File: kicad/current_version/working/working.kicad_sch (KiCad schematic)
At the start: 4 parts, among them IC1 imsp10mpump21rs2227

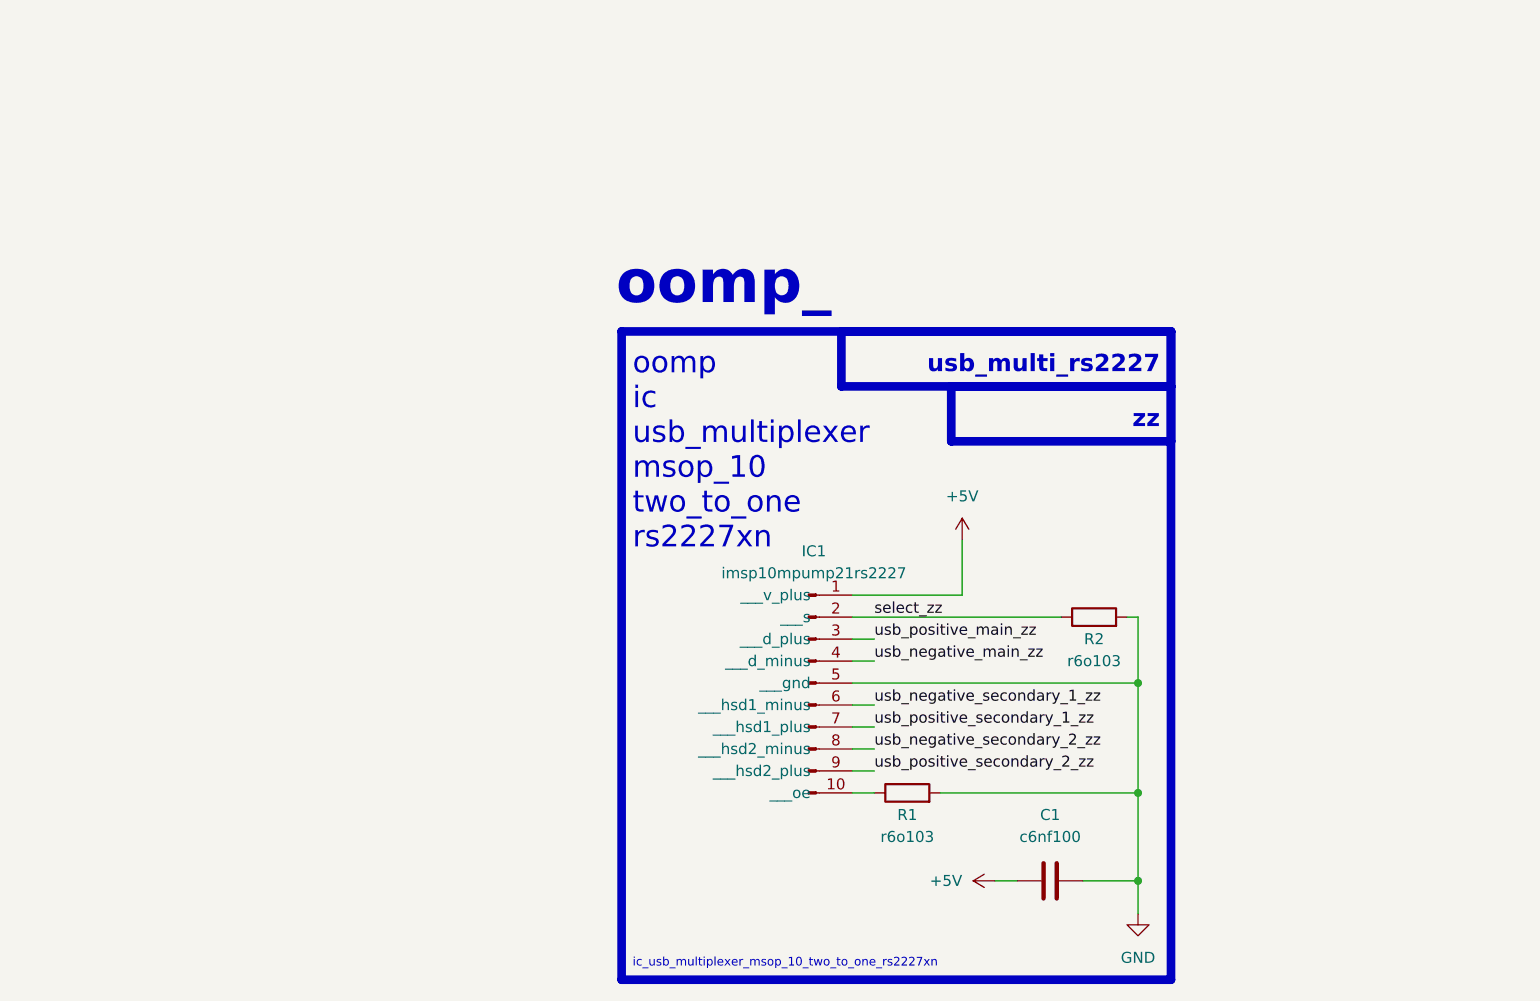
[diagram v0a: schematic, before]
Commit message: initial
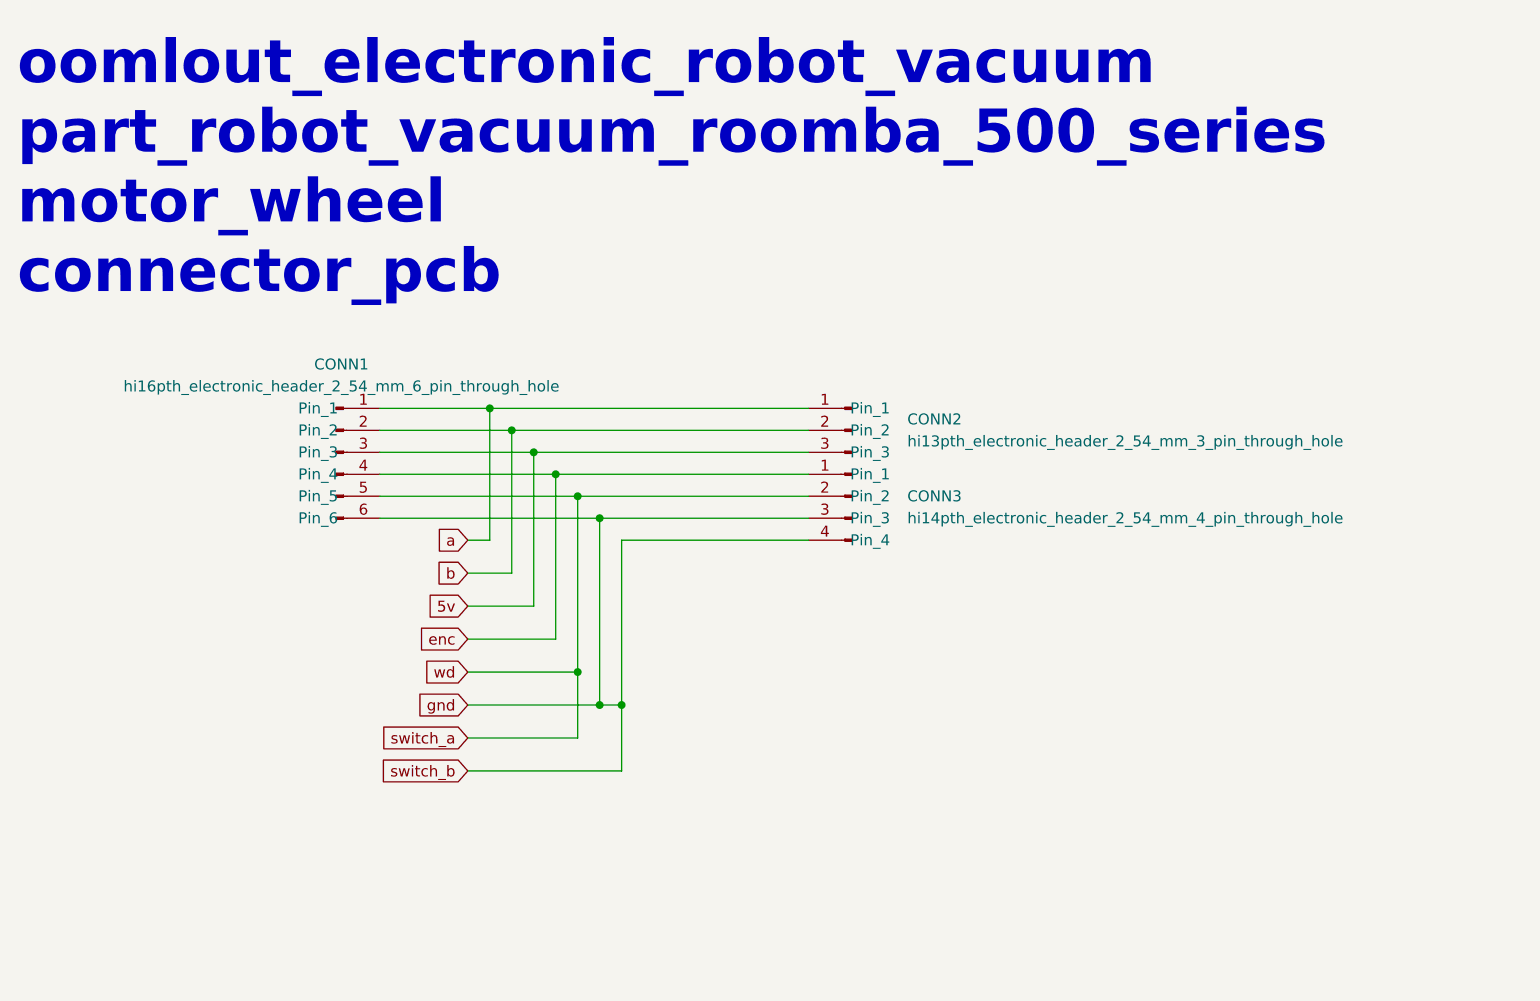
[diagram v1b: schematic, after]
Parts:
- removed C1: c6nf100, oomlout_oomp_part_footprints:c6nf100_electronic_capacitor_0603_100_nano_farad, symbol oomlout_oomp_part_symbols:c6nf100_electronic_capacitor_0603_100_nano_farad
- removed IC1: imsp10mpump21rs2227, oomlout_oomp_part_footprints:imsp10mpump21rs2227_electronic_ic_msop_10_multiplexer_usb_multiplexer_two_to_one_jiangsu_r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, symbol oomlout_oomp_part_symbols:imsp10mpump21rs2227_electronic_ic_msop_10_multiplexer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
- removed R1, R2: r6o103, oomlout_oomp_part_footprints:r6o103_electronic_resistor_0603_10000_ohm, symbol oomlout_oomp_part_symbols:r6o103_electronic_resistor_0603_10000_ohm
- added CONN1: hi16pth_electronic_header_2_54_mm_6_pin_through_h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, oomlout_oomp_part_footprints:hi16pth_electronic_header_2_54_mm_6_pin_through_hole, symbol oomp:hi16pth_electronic_header_2_54_mm_6_pin_through_hole
- added CONN2: hi13pth_electronic_header_2_54_mm_3_pin_through_h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, oomlout_oomp_part_footprints:hi13pth_electronic_header_2_54_mm_3_pin_through_hole, symbol oomp:hi13pth_electronic_header_2_54_mm_3_pin_through_hole
- added CONN3: hi14pth_electronic_header_2_54_mm_4_pin_through_h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, oomlout_oomp_part_footprints:hi14pth_electronic_header_2_54_mm_4_pin_through_hole, symbol oomp:hi14pth_electronic_header_2_54_mm_4_pin_through_hole
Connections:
- new net 5v: CONN1.3 (Pin_3), CONN2.3 (Pin_3)
- new net a: CONN1.1 (Pin_1), CONN2.1 (Pin_1)
- new net b: CONN1.2 (Pin_2), CONN2.2 (Pin_2)
- new net enc: CONN1.4 (Pin_4), CONN3.1 (Pin_1)
- new net gnd: CONN1.6 (Pin_6), CONN3.3 (Pin_3), CONN3.4 (Pin_4)
- new net switch_a: CONN1.5 (Pin_5), CONN3.2 (Pin_2)
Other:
- note added: "oomlout_electronic_robot_vacuum part_robot_vacuum_roomba_500_series motor_wheel connector_pcb"
- note removed: "ic_usb_multiplexer_msop_10_two_to_one_rs2227xn"
- note removed: "oomp ic usb_multiplexer msop_10 two_to_one rs2227xn"
- note removed: "oomp_"
- note removed: "usb_multi_rs2227"
- note removed: "zz"
